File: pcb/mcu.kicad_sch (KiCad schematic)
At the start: 27 parts, among them SW1 PTS810, SW2 PTS810, U1 RP2040, U2 W25Q16JVSS, Y1 ABM8-272-T3

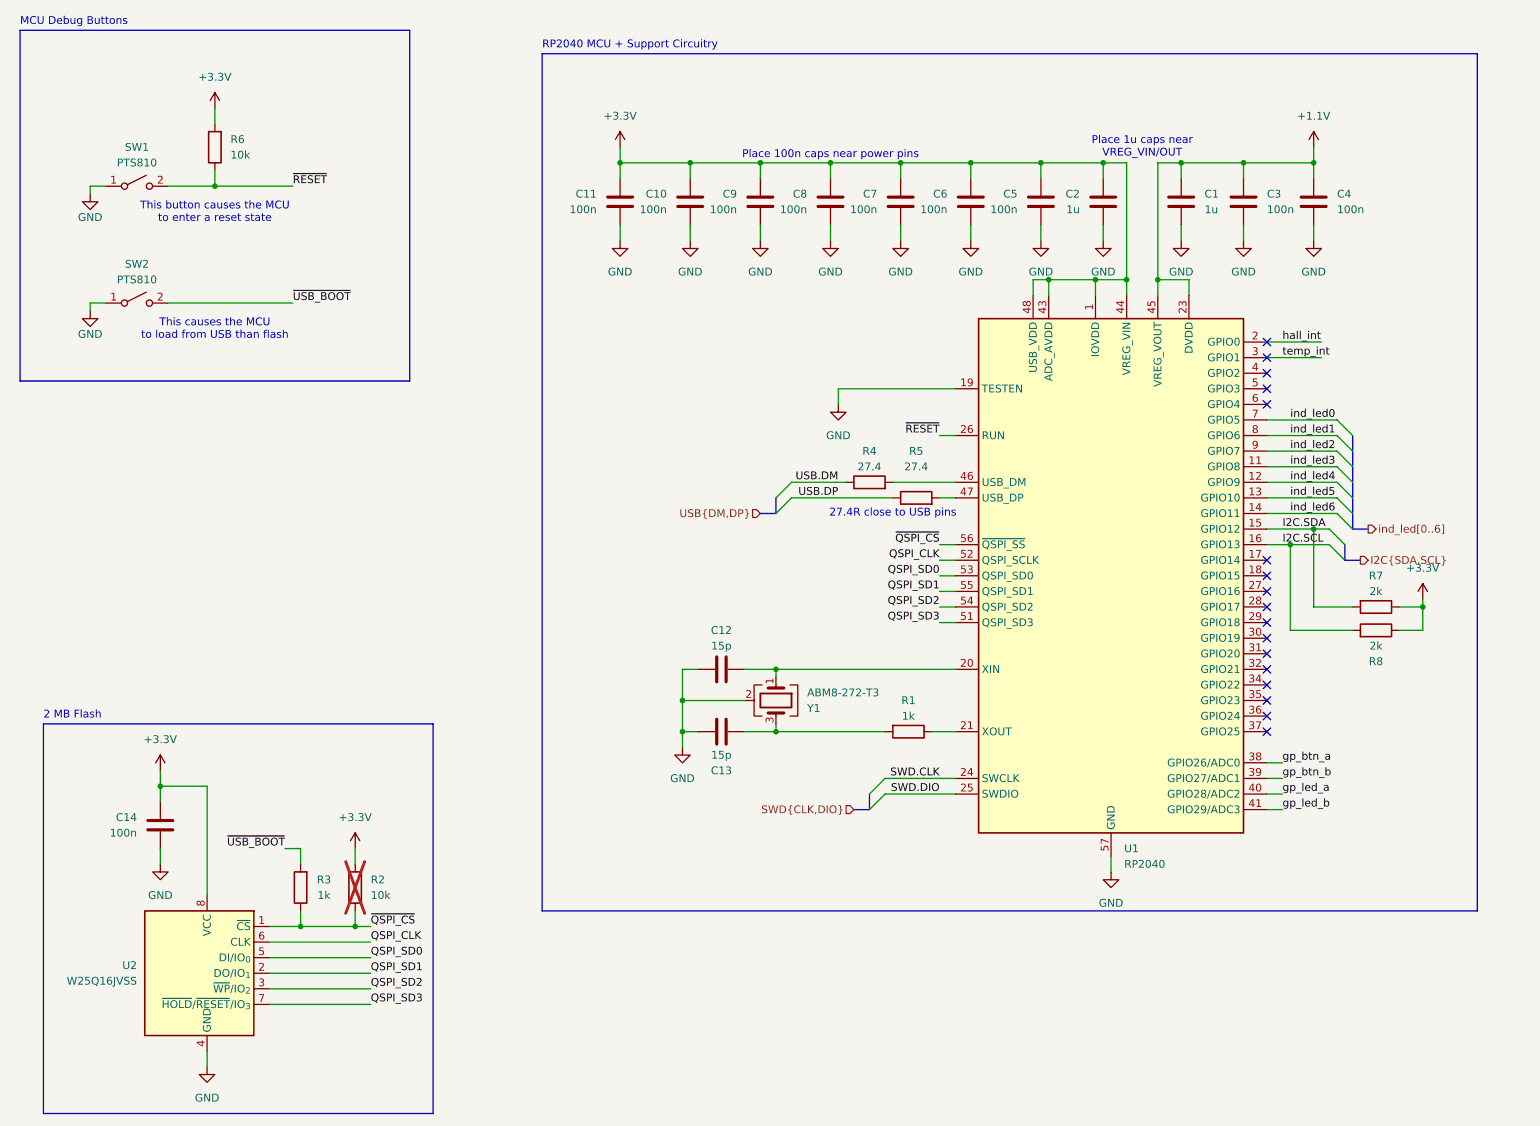
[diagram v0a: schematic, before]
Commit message: add top level schem and cleanup
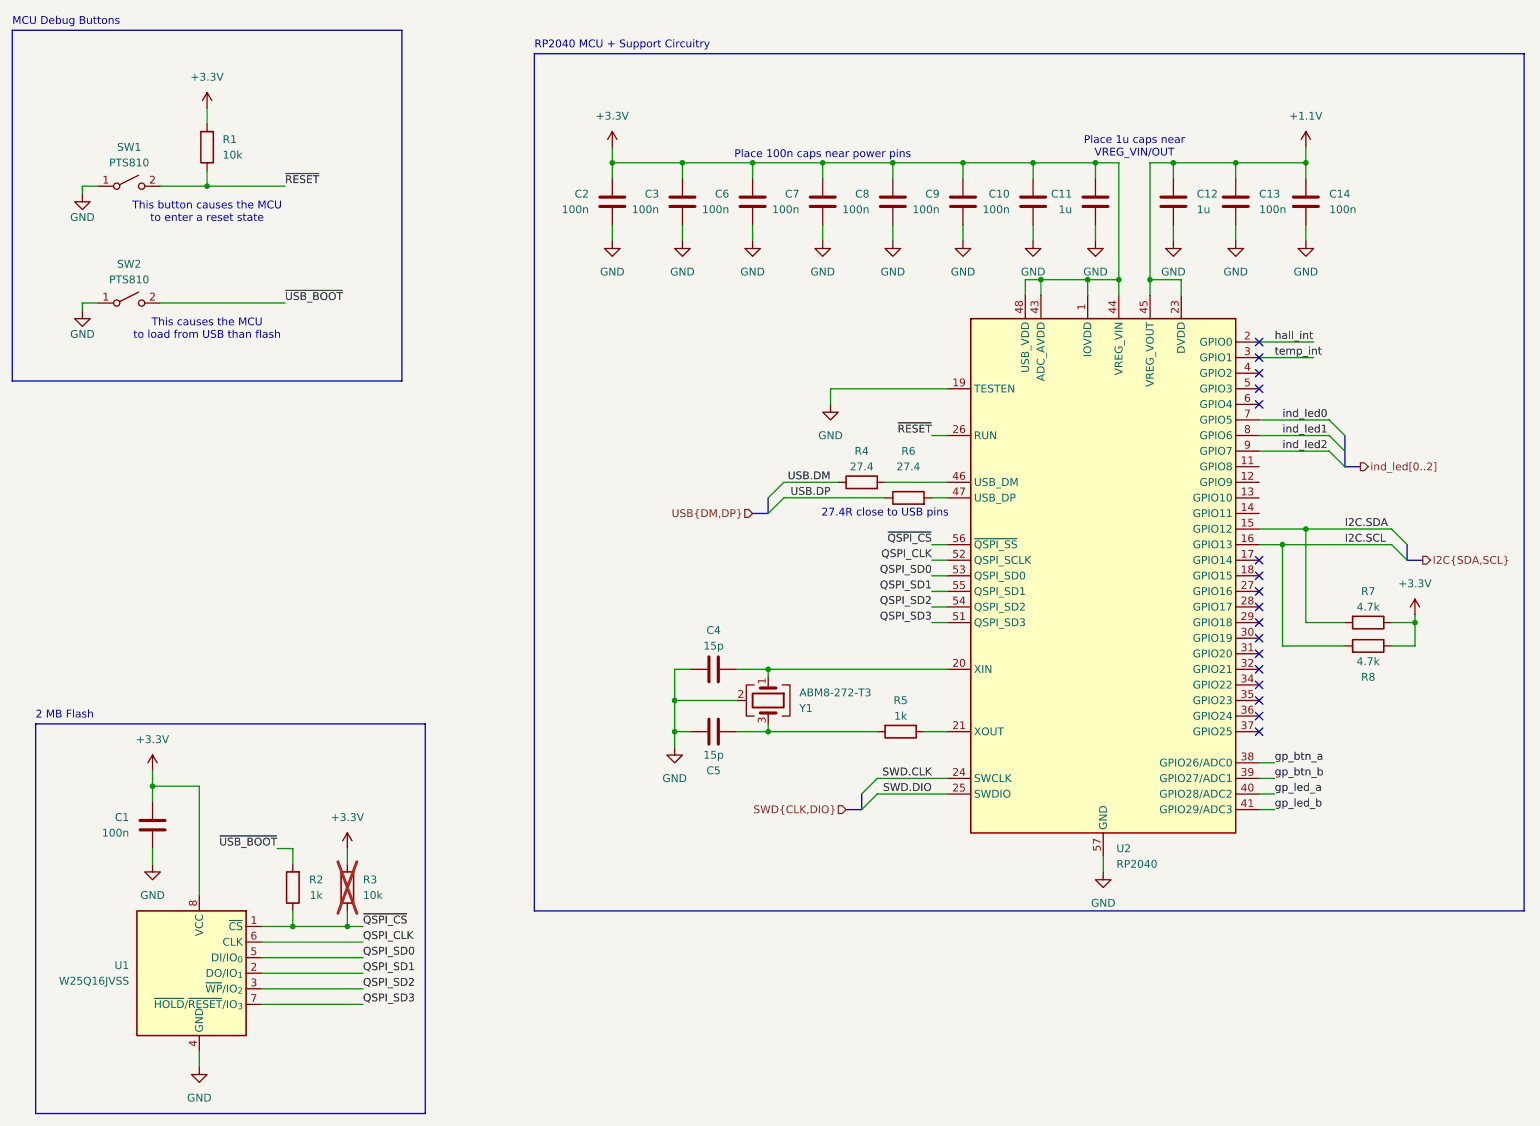
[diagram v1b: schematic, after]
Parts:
- removed U1: RP2040, Package_DFN_QFN:QFN-56-1EP_7x7mm_P0.4mm_EP3.2x3.2mm, symbol MCU_RaspberryPi:RP2040
- removed U2: W25Q16JVSS, Package_SO:SOIC-8_5.3x5.3mm_P1.27mm, symbol Memory_Flash:W25Q16JVSS
- added U1: W25Q16JVSS, Package_SO:SOIC-8_5.3x5.3mm_P1.27mm, symbol Memory_Flash:W25Q16JVSS
- added U2: RP2040, Package_DFN_QFN:QFN-56-1EP_7x7mm_P0.4mm_EP3.2x3.2mm, symbol MCU_RaspberryPi:RP2040
- C1, C2: value 1u -> 100n; Manufacturer P/N GRM155Z71A105KE01J -> (none); Vendor DigiKey -> (none); Vendor P/N 490-GRM155Z71A105KE01JCT-ND -> (none)
- C11: value 100n -> 1u; Manufacturer P/N (none) -> GRM155Z71A105KE01J; Vendor (none) -> DigiKey; Vendor P/N (none) -> 490-GRM155Z71A105KE01JCT-ND
- C12: value 15p -> 1u; Manufacturer P/N GRM1555C1H150JA01D -> GRM155Z71A105KE01J; Vendor P/N 490-5888-1-ND -> 490-GRM155Z71A105KE01JCT-ND
- C13: value 15p -> 100n; Manufacturer P/N GRM1555C1H150JA01D -> (none); Vendor DigiKey -> (none); Vendor P/N 490-5888-1-ND -> (none)
- C4, C5: value 100n -> 15p; Manufacturer P/N (none) -> GRM1555C1H150JA01D; Vendor (none) -> DigiKey; Vendor P/N (none) -> 490-5888-1-ND
- R1: value 1k -> 10k; Manufacturer P/N RC0402FR-071KL -> RC0402FR-0710KL; Vendor P/N 311-1.00KLRCT-ND -> 311-10.0KLRCT-ND
- R2: value 10k -> 1k; Manufacturer P/N RC0402FR-0710KL -> RC0402FR-071KL; Vendor P/N 311-10.0KLRCT-ND -> 311-1.00KLRCT-ND; now fitted
- R3: value 1k -> 10k; Manufacturer P/N RC0402FR-071KL -> RC0402FR-0710KL; Vendor P/N 311-1.00KLRCT-ND -> 311-10.0KLRCT-ND; now not fitted
- R5: value 27.4 -> 1k; Manufacturer P/N RC0402FR-0727R4L -> RC0402FR-071KL; Vendor P/N YAG3085CT-ND -> 311-1.00KLRCT-ND
- R6: value 10k -> 27.4; Manufacturer P/N RC0402FR-0710KL -> RC0402FR-0727R4L; Vendor P/N 311-10.0KLRCT-ND -> YAG3085CT-ND
- R7, R8: value 2k -> 4.7k
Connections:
- net +1.1V: now also C12.1, C13.1, C14.1, U2.23 (DVDD), U2.45 (VREG_VOUT), U2.50 (DVDD); no longer C1.1, C3.1, C4.1
- net +3.3V: now also C1.1, C3.1, R1.2, R3.1, U1.8 (VCC), U2.1 (IOVDD), U2.10 (IOVDD), U2.22 (IOVDD), U2.33 (IOVDD), U2.42 (IOVDD), U2.43 (ADC_AVDD), U2.44 (VREG_VIN), U2.48 (USB_VDD), U2.49 (IOVDD); no longer C14.1, C5.1, R2.1, R6.2
- net GND: now also C12.2, C13.2, C4.1, C5.1, U1.4 (GND), U2.19 (TESTEN), U2.57 (GND); no longer C12.1, C13.1, C4.2, C5.2
- net I2C.SCL: now also U2.16 (GPIO13)
- net I2C.SDA: now also U2.15 (GPIO12)
- net QSPI_CLK: now also U1.6 (CLK), U2.52 (QSPI_SCLK)
- net QSPI_SD0: now also U1.5 (DI/IO_{0}), U2.53 (QSPI_SD0)
- net QSPI_SD1: now also U1.2 (DO/IO_{1}), U2.55 (QSPI_SD1)
- net QSPI_SD2: now also U1.3 (~{WP}/IO_{2}), U2.54 (QSPI_SD2)
- net QSPI_SD3: now also U1.7 (~{HOLD}/~{RESET}/IO_{3}), U2.51 (QSPI_SD3)
- net SWD.CLK: now also U2.24 (SWCLK)
- net SWD.DIO: now also U2.25 (SWDIO)
- net USB.DP: now also R6.1; no longer R5.1
- net gp_btn_a: now also U2.38 (GPIO26/ADC0)
- net gp_btn_b: now also U2.39 (GPIO27/ADC1)
- net gp_led_a: now also U2.40 (GPIO28/ADC2)
- net gp_led_b: now also U2.41 (GPIO29/ADC3)
- net hall_int: now also U2.2 (GPIO0)
- net ind_led0: now also U2.7 (GPIO5)
- net ind_led1: now also U2.8 (GPIO6)
- net ind_led2: now also U2.9 (GPIO7)
- net temp_int: now also U2.3 (GPIO1)
- net ~{QSPI_CS}: now also R2.1, R3.2, U1.1 (~{CS}), U2.56 (~{QSPI_SS}); no longer R2.2, R3.1
- net ~{RESET}: now also R1.1, U2.26 (RUN); no longer R6.1
- net ~{USB_BOOT}: now also R2.2; no longer R3.2
- net at Y1.1: now also C4.2, U2.20 (XIN); no longer C12.2
- net at R4.2: now also U2.46 (USB_DM)
- net at R5.2: now also C5.2, Y1.3
- new net: R5.1, U2.21 (XOUT)
- new net: R6.2, U2.47 (USB_DP)
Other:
- title: (none) -> MCU
